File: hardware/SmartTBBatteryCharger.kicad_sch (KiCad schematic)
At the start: 217 parts, among them J1 XT60_MALE, J2 XT60_MALE, J3 XT60_MALE, J4 XT60_MALE, J5 XT60_MALE, J6 XT60_MALE, J7 Conn_SWD, J8 Conn_01x02, Q1 BSC070N10NS5, Q2 BSC070N10NS5, Q3 BSC070N10NS5, Q4 BSC070N10NS5, Q5 BSC070N10NS5, Q6 BSC070N10NS5, U1 RY8411, U10 INA240A1PW, U11 UCC27517, U12 UCC27517, U13 UCC27517, U14 INA240A1PW, U15 INA240A1PW, U16 INA240A1PW, U2 RS3236, U3 RY8411, U4 STM32G474RBTx, U5 INA240A1PW, U6 UCC27517, U7 UCC27517, U8 INA240A1PW, U9 UCC27517, Y1 Crystal_GND24

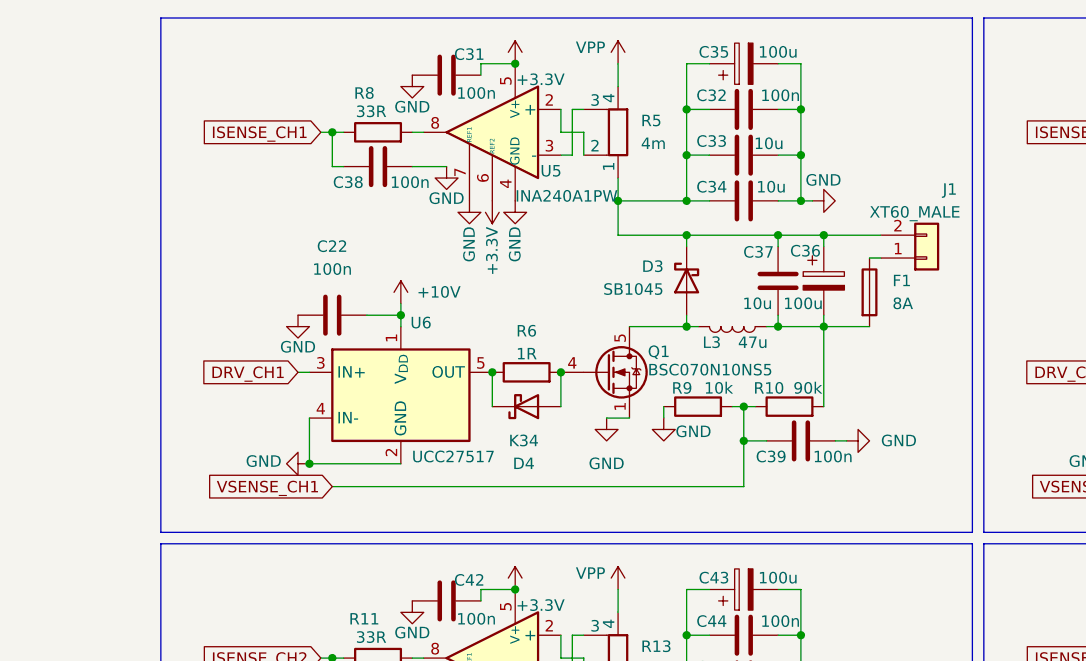
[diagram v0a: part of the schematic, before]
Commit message: Update Hardware
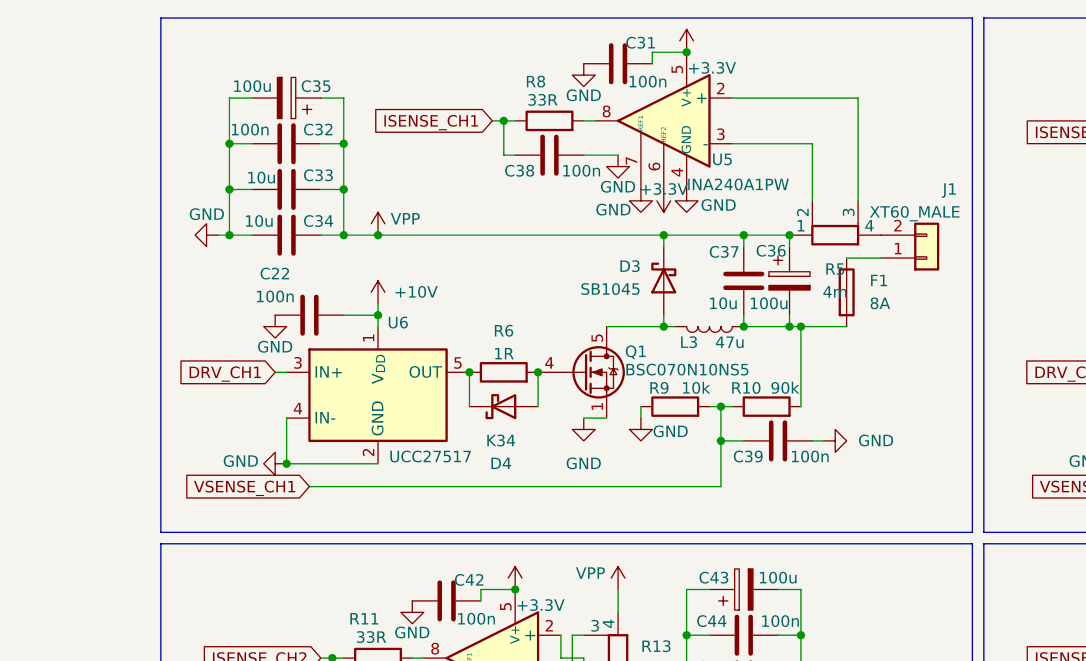
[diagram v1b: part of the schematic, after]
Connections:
- net VPP: now also C32.1, C33.1, C34.1, C35.1, C36.1, C37.1, D3.1 (K), R5.1; no longer R5.4
- net at U5.2 (+): now also R5.3; no longer R5.2
- net at U5.3 (-): now also R5.2; no longer R5.3
- new net: J1.2 (Pin_2), R5.4
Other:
- moved on the sheet: C22, C31, C32, C33, C34, C35, C36, C37, C38, C39, D3, D4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
